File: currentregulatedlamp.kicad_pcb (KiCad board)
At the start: 2 copper layers, 9 parts, among them J1 Conn_01x12, J2 Conn_01x16, U1 TPS54308DDC

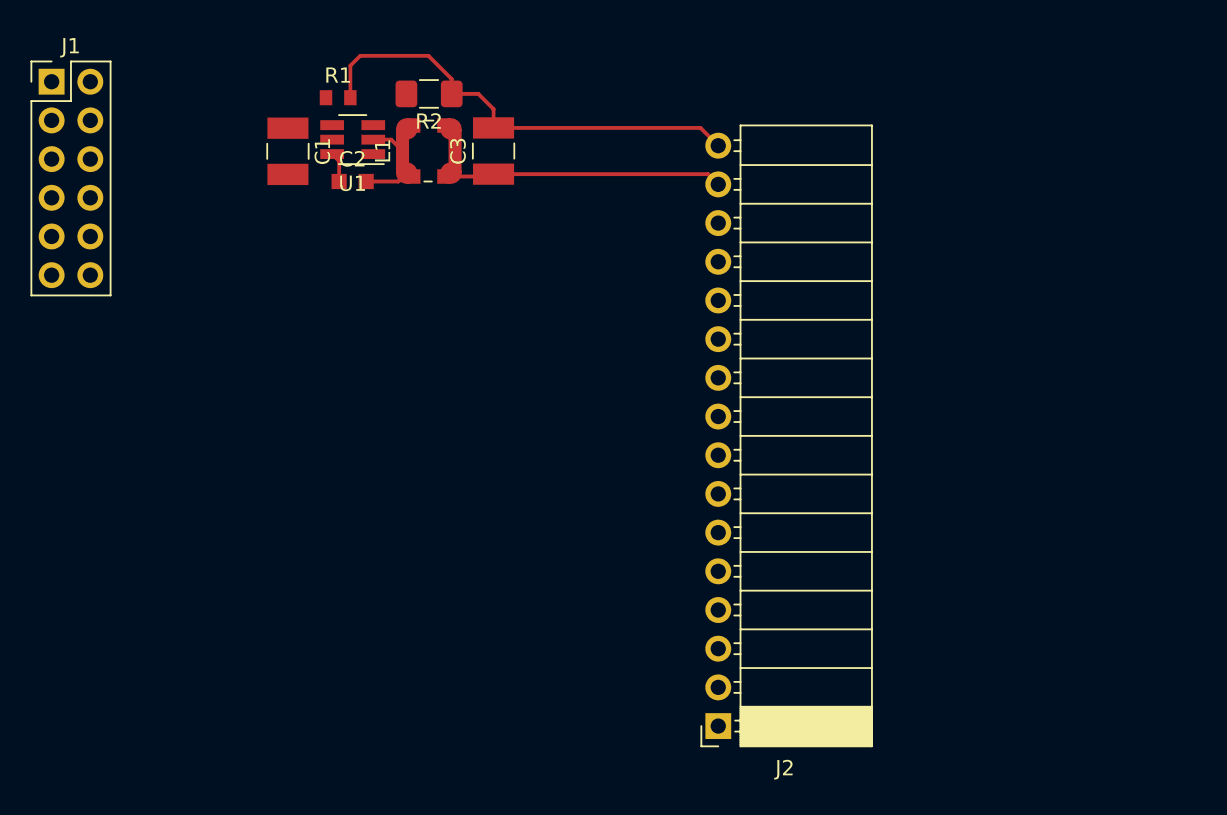
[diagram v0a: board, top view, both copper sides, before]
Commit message: Schematic replication
decided on path for replicating current regulator
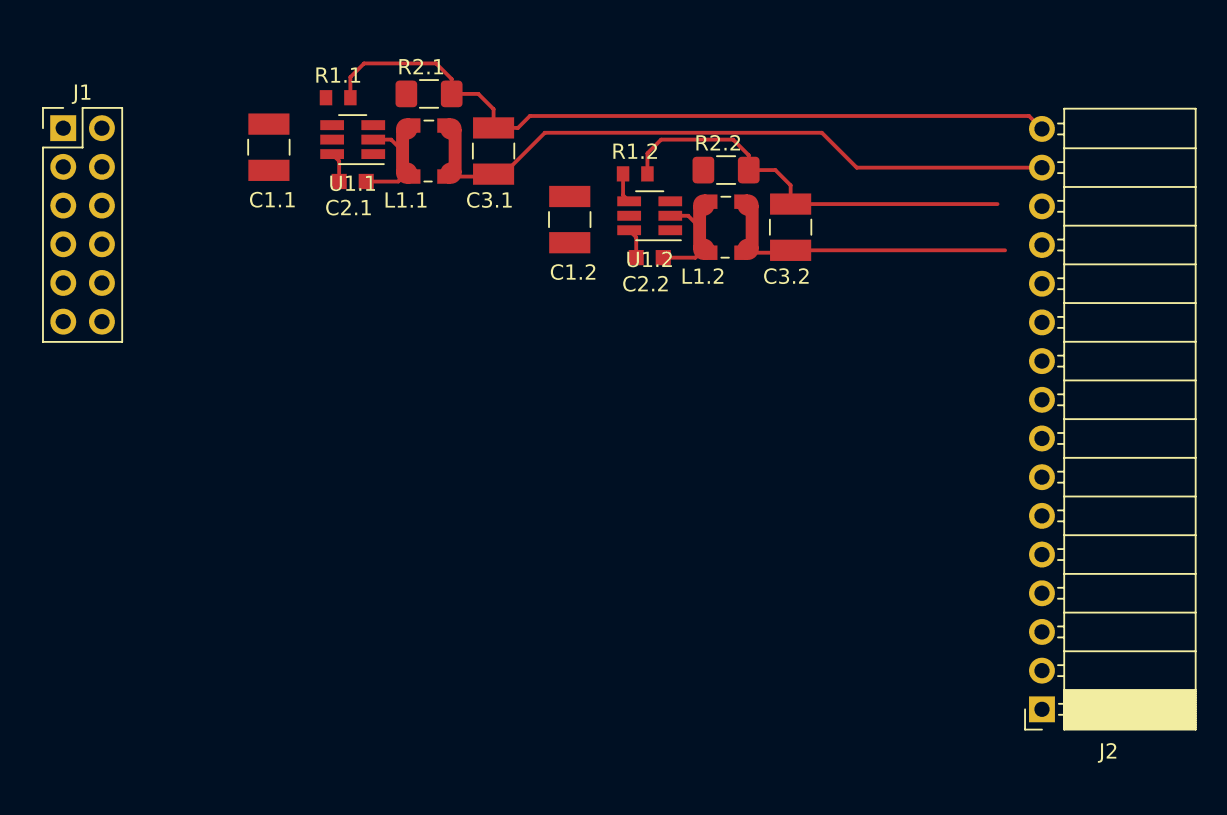
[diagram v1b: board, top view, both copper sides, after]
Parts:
- added C1.2: C, Capacitor_SMD:C_1210_3225Metric_Pad1.39x2.70mm_HandSolder, F.Cu at (65.0, 53.5)
- added C2.2: 100n/50V, Capacitor_SMD:C_0603_1608Metric_Pad0.99x1.00mm_HandSolder, F.Cu at (70.2, 56.0)
- added C3.2: C, Capacitor_SMD:C_1210_3225Metric_Pad1.39x2.70mm_HandSolder, F.Cu at (79.5, 54.0)
- added L1.2: L, Inductor_SMD:L_Wuerth_WE-TPC-3816, F.Cu at (75.2, 54.0)
- added R1.2: R, Resistor_SMD:R_0603_1608Metric, F.Cu at (69.3, 50.5)
- added R2.2: R, Resistor_SMD:R_1206_3216Metric_Pad1.42x1.75mm_HandSolder, F.Cu at (75.3, 50.2)
- added U1.2: TPS54308DDC, Package_TO_SOT_SMD:SOT-23-6_Handsoldering, F.Cu at (70.2, 53.2)
- moved J2 21.3 mm to (96.0, 85.7)
- moved J1 3.14 mm to (31.8, 47.5)
- moved C1.1 1.28 mm to (45.2, 48.8)
- renumbered C1 to C1.1, C2 to C2.1, C3 to C3.1, L1 to L1.1, R1 to R1.1, R2 to R2.1, U1 to U1.1
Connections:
- J1 pad 6: Net-(J1-Pad6) -> /LED_2/DIM
- J2 pad 15: /TPS54200/LED+ -> Net-(J2-Pad15)
- J2 pad 16: /TPS54200/LED- -> Net-(J2-Pad16)
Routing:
- net /LED-: track 0.00 -> 50.8 mm
- net /LED+: track 0.00 -> 43.5 mm
- net /TPS54200/LED-: track 30.3 -> 0.00 mm
- net /LED_2/LED-: track 0.00 -> 27.8 mm
- net /TPS54200/LED+: track 20.4 -> 0.00 mm
- net /LED_2/LED+: track 0.00 -> 19.5 mm
- net /LED_2/SW: track 0.00 -> 5.13 mm
- net /LED_2/BOOT: track 0.00 -> 1.99 mm
- net /LED_2/FB: track 0.00 -> 1.97 mm
